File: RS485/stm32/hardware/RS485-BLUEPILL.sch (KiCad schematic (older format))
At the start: 6 parts, among them P1 CONN_01X03, P2 CONN_01X02, U1 BLUE-PILL, U2 MAX485/SN75176

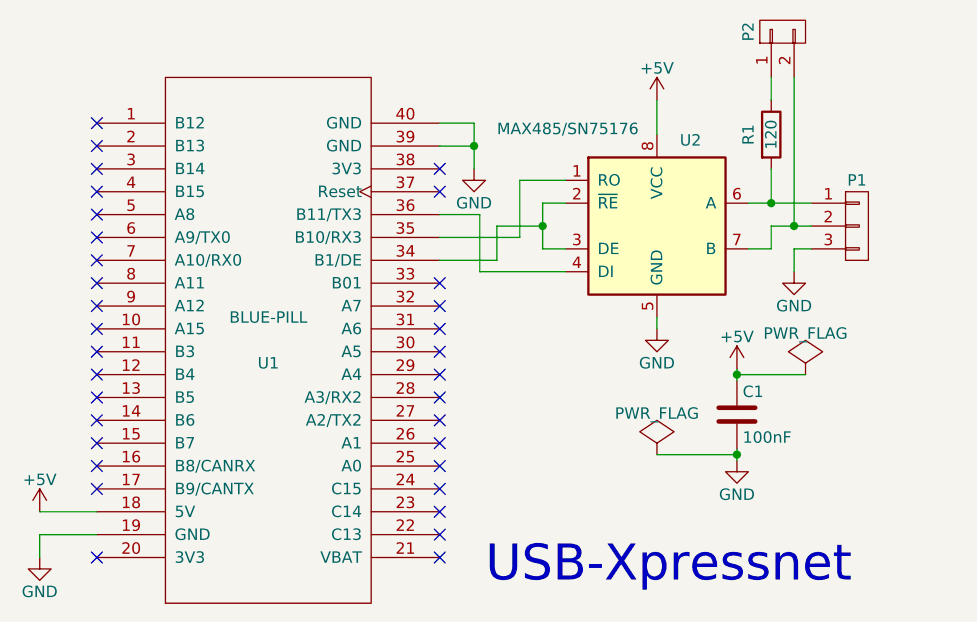
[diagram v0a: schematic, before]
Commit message: RS422 idea
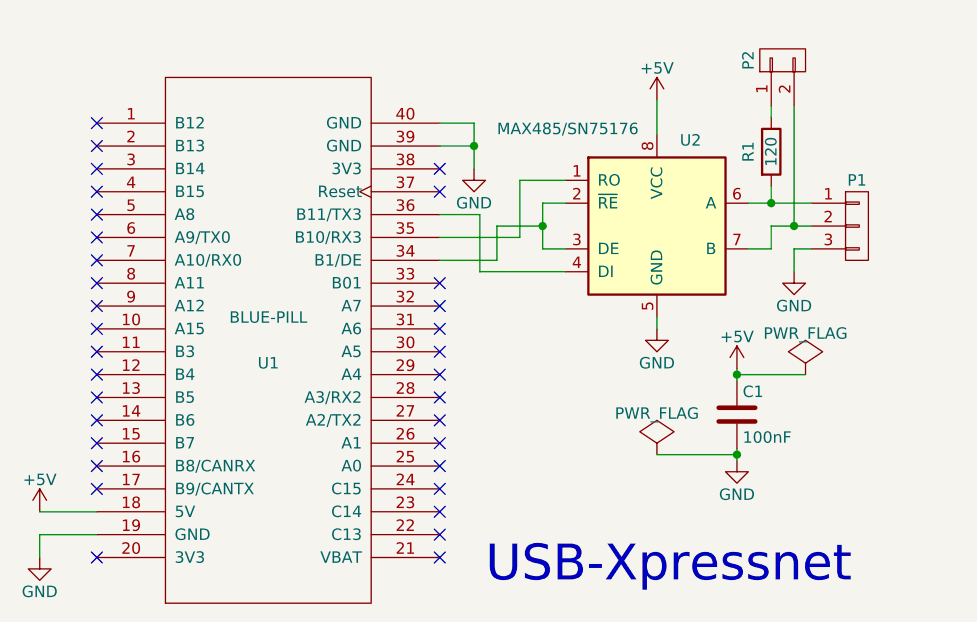
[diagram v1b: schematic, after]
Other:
- moved on the sheet: P2, R1
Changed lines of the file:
@@
 L R R1
 U 1 1 59CCE923
-P 7150 2700
-F 0 "R1" V 7050 2700 50  0000 C CNN
-F 1 "120" V 7150 2700 50  0000 C CNN
-F 2 "" V 7080 2700 50  0000 C CNN
-F 3 "" H 7150 2700 50  0000 C CNN
-	1    7150 2700
+P 7150 2775
+F 0 "R1" V 7050 2775 50  0000 C CNN
+F 1 "120" V 7150 2775 50  0000 C CNN
+F 2 "" V 7080 2775 50  0000 C CNN
+F 3 "" H 7150 2775 50  0000 C CNN
+	1    7150 2775
 	1    0    0    -1
 $EndComp
@@
 L CONN_01X02 P2
 U 1 1 59CCE9B8
-P 7200 2250
-F 0 "P2" H 7200 2400 50  0000 C CNN
-F 1 "CONN_01X02" V 7300 2250 50  0001 C CNN
-F 2 "" H 7200 2250 50  0000 C CNN
-F 3 "" H 7200 2250 50  0000 C CNN
-	1    7200 2250
+P 7200 2375
+F 0 "P2" H 7200 2525 50  0000 C CNN
+F 1 "CONN_01X02" V 7300 2375 50  0001 C CNN
+F 2 "" H 7200 2375 50  0000 C CNN
+F 3 "" H 7200 2375 50  0000 C CNN
+	1    7200 2375
 	0    -1   -1   0
 $EndComp
@@
 	6650 3500 6650 3550
 Wire Wire Line
-	7050 3000 7325 3000
+	7050 3000 7150 3000
+Wire Wire Line
+	7150 3000 7325 3000
 Wire Wire Line
 	7150 3200 7150 3100
 Wire Wire Line
-	7150 3100 7325 3100
+	7150 3100 7250 3100
+Wire Wire Line
+	7250 3100 7325 3100
 Wire Wire Line
 	7150 3200 7050 3200
 Wire Wire Line
-	7150 3000 7150 2850
+	7150 3000 7150 2925
 Connection ~ 7150 3000
 Wire Wire Line
-	7150 2450 7150 2550
+	7150 2575 7150 2625
 Wire Wire Line
-	7250 2450 7250 3100
+	7250 2575 7250 3100
 Connection ~ 7250 3100
 Wire Wire Line
-	7000 3725 7000 3775
+	7000 3725 7000 3750
 Wire Wire Line
-	7000 4075 7000 4125
+	7000 3750 7000 3775
+Wire Wire Line
+	7000 4075 7000 4100
+Wire Wire Line
+	7000 4100 7000 4125
 Wire Wire Line
 	4200 4450 3950 4450
@@
 	5700 2650 5850 2650
 Wire Wire Line
-	5850 2650 5850 2850
+	5850 2650 5850 2750
+Wire Wire Line
+	5850 2750 5850 2850
 Wire Wire Line
 	5850 2750 5700 2750
@@
 	6250 3000 6150 3000
 Wire Wire Line
-	6150 3000 6150 3200
+	6150 3000 6150 3100
+Wire Wire Line
+	6150 3100 6150 3200
 Wire Wire Line
 	6150 3200 6250 3200
